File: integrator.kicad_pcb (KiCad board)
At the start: 4 copper layers, 65.5 x 117 mm, 23 parts, among them J1 SJ-3524-SMT, J2 SJ-3524-SMT, SW1 EVQP40B3M, SW2 EVQP40B3M, U1 Teensy3.2, U2 ICM-20600

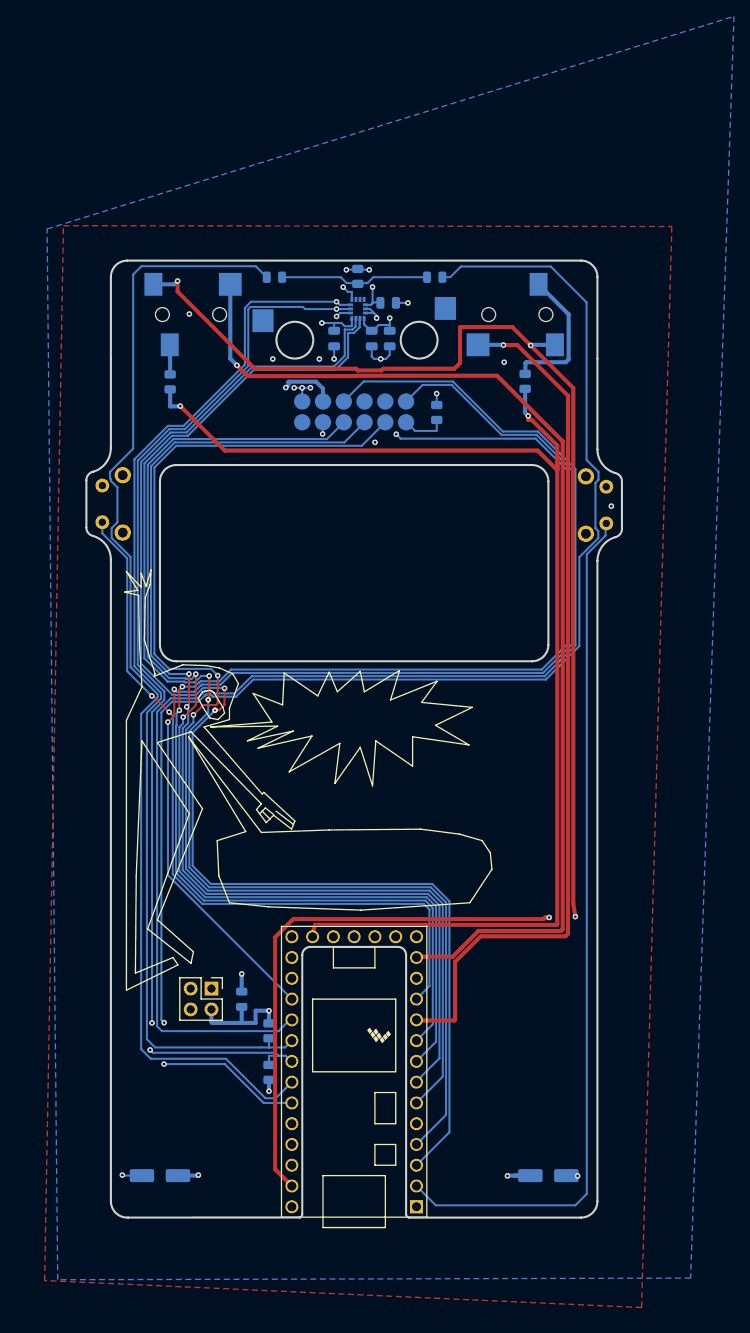
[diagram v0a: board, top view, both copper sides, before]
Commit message: evt4 pcb layout
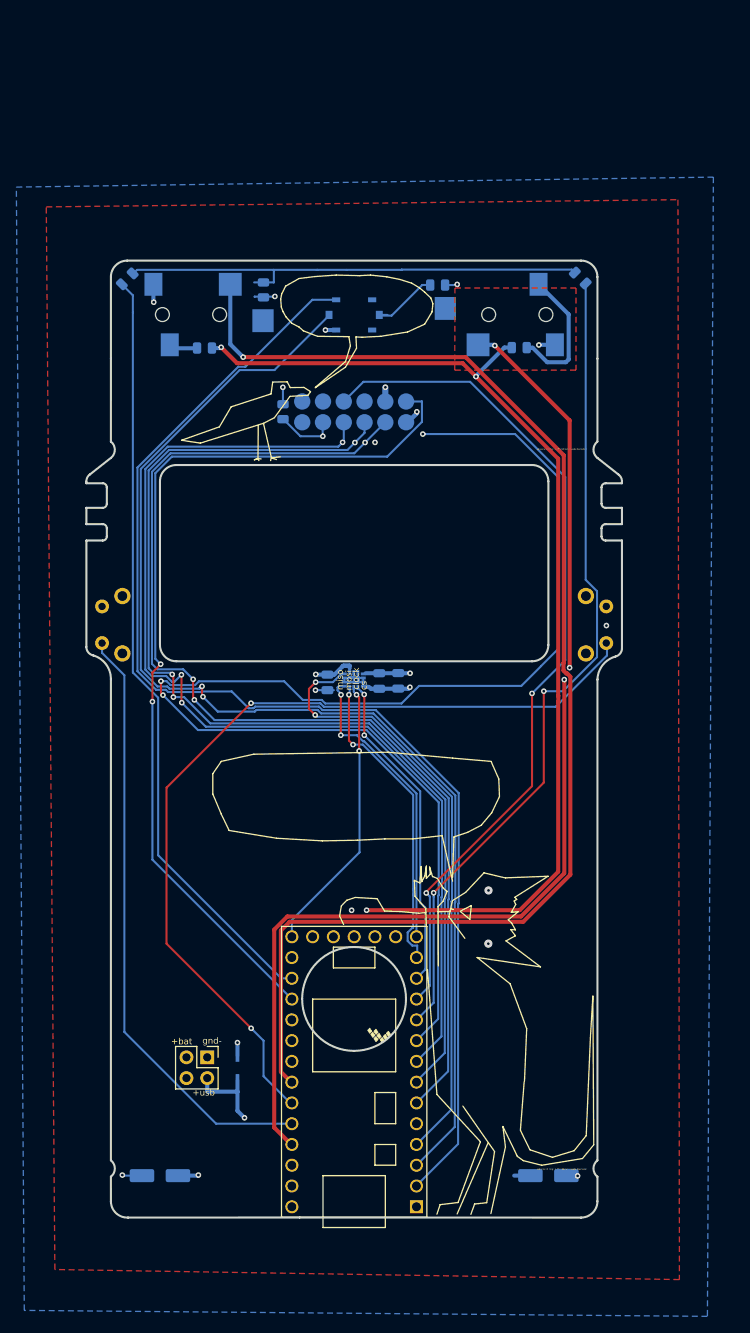
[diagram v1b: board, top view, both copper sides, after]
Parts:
- removed C5: 0.1uf, Capacitor_SMD:C_0805_2012Metric
- removed R3: 4.7k, Resistor_SMD:R_0805_2012Metric
- removed U2: ICM-20600, PQFN50P250X300X97-14N
- added IMU: ICM-42605, ICM-42605:PQFN50P300X250X97-14N, B.Cu at (154.0, 95.3)
- added NON       STOP: SW_Push_LED, TL3215AF160BQ:E-Switch-N326000-0-0-0, B.Cu at (154.0, 50.6)
- D1: footprint Diode_SMD:D_0805_2012Metric -> Diode_SMD:D_SOD-323
- R2: value 4.7k -> 47
- moved R2 98.5 mm to (164.3, 47.0), turned to 180 degrees
- moved C1 47.0 mm to (150.8, 95.6), turned to 90 degrees
- moved C2 41.9 mm to (157.1, 95.4)
- moved C3 41.9 mm to (159.4, 95.4)
- moved R6 18.8 mm to (145.3, 62.5)
- moved LED1 18.0 mm to (126.3, 46.2), turned to 225 degrees
- moved LED2 17.8 mm to (181.7, 46.1), turned to 315 degrees
- moved SW2 14.8 mm to (128.3, 88.5)
- moved SW1 14.6 mm to (179.8, 88.5)
- moved R1 11.7 mm to (143.0, 47.6), turned to 270 degrees
- moved D1 8.42 mm to (139.8, 142.7)
- moved REF** 8.42 mm to (136.1, 141.4)
- moved R4 5.90 mm to (135.7, 54.7), turned to 180 degrees
- moved R5 4.19 mm to (174.2, 54.6), turned to 180 degrees
- renumbered C6 to DUM, C4 to DUM_R
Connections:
- POGO1 pad 10: Net-(POGO1-Pad10) -> Earth
- POGO1 pad 11: Net-(POGO1-Pad11) -> /po_batt
- POGO1 pad 2: Earth -> Net-(POGO1-Pad2)
- POGO1 pad 4: /po_batt -> Net-(POGO1-Pad4)
- R2 pad 1: /+3.3v -> Earth
- R2 pad 2: /i2c_clk -> Net-(R2-Pad2)
- R6 pad 1: Net-(POGO1-Pad11) -> /po_reset
- R6 pad 2: /po_reset -> Earth
- REF** pad 1: (no net) -> Earth
- SW1 pad 2: /l_button -> /sw1
- SW2 pad 1: /r_button -> /sw2
- U1 pad 10: /r_sync_out -> /led2
- U1 pad 11: /r_button -> /po_wake
- U1 pad 12: Net-(U1-Pad12) -> /spi_cs
- U1 pad 13: /l_sync_out -> /spi_mosi
- U1 pad 14: Net-(U1-Pad14) -> /spi_miso
- U1 pad 2: /l_button -> /nonstop_sw
- U1 pad 20: Net-(U1-Pad20) -> /spi_clock
- U1 pad 22: Net-(U1-Pad22) -> /led1
- U1 pad 24: /po_wake -> Net-(U1-Pad24)
- U1 pad 25: /i2c_sda -> Net-(U1-Pad25)
- U1 pad 26: /i2c_clk -> Net-(U1-Pad26)
- U1 pad 27: /led1 -> /l_sync_out
- U1 pad 28: /led2 -> /sw1
- U1 pad 29: Net-(U1-Pad29) -> /sw2
- U1 pad 3: /amu_sync -> /nonstop_led
- U1 pad 30: Net-(U1-Pad30) -> /r_sync_out
- U1 pad 4: /amu_int2 -> /imu_int1
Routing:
- net /a_gnd: track 275.8 -> 4.28 mm, vias 4 -> 3
- net /amu_sync: track 163.6 -> 0.00 mm, vias 2 -> 0
- net /amu_int2: track 158.1 -> 0.00 mm, vias 2 -> 0
- net /nonstop_sw: track 0.00 -> 153.2 mm
- net /nonstop_led: track 0.00 -> 149.0 mm, vias 0 -> 2
- net /+3.3v: track 285.0 -> 148.6 mm, vias 7 -> 4
- net /i2c_clk: track 132.3 -> 0.00 mm, vias 3 -> 0
- net /i2c_sda: track 131.2 -> 0.00 mm, vias 1 -> 0
- net /sw1: track 0.00 -> 106.8 mm, vias 0 -> 2
- net /l_button: track 105.1 -> 0.00 mm
- net /r_button: track 91.5 -> 0.00 mm, vias 2 -> 0
- net /led2: track 179.3 -> 101.1 mm
- net /sw2: track 0.00 -> 73.8 mm
- net /imu_int1: track 0.00 -> 73.8 mm, vias 0 -> 2
- net /po_wake: track 165.6 -> 104.7 mm, vias 0 -> 2
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- added copper zone on In2.Cu, net /+3.3v
- added copper zone on F.Cu, net /a_gnd
- removed copper zone on In2.Cu, net Earth
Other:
- outline, holes or cut-outs redrawn
- board text added: "+bat"
- board text added: "+usb"
- board text added: "F_U_CN_RD UR_BKWDS"
- board text added: "MSL Pocket Integrator evt4 Summer 2021"
- board text added: "NON STOP"
- board text added: "OUT"
- board text added: "PO INPUT"
- board text added: "TO WORLD"
- board text added: "clock"
- board text added: "cs"
- board text added: "gnd-"
- board text added: "miso"
- board text added: "mosi"
- board text added: "silicone O ring: 1.75”/44mm inside diameter"
- board text added: "• attach with 2 O rings 1.75”/44mm I.D. • connect either output to PO input • set PO sync mode to SY4 • shake it like a polaroid picture"
- board text removed: "MSL Pocket Integrator rev1 Spring 2021"
- board text removed: "• attach with bolts, glue or duct tape • connect either output to PO input • set PO sync mode to SY4 • unplug to let PO sleep • repetition is a form of change"
